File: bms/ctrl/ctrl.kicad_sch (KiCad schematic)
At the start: 72 parts

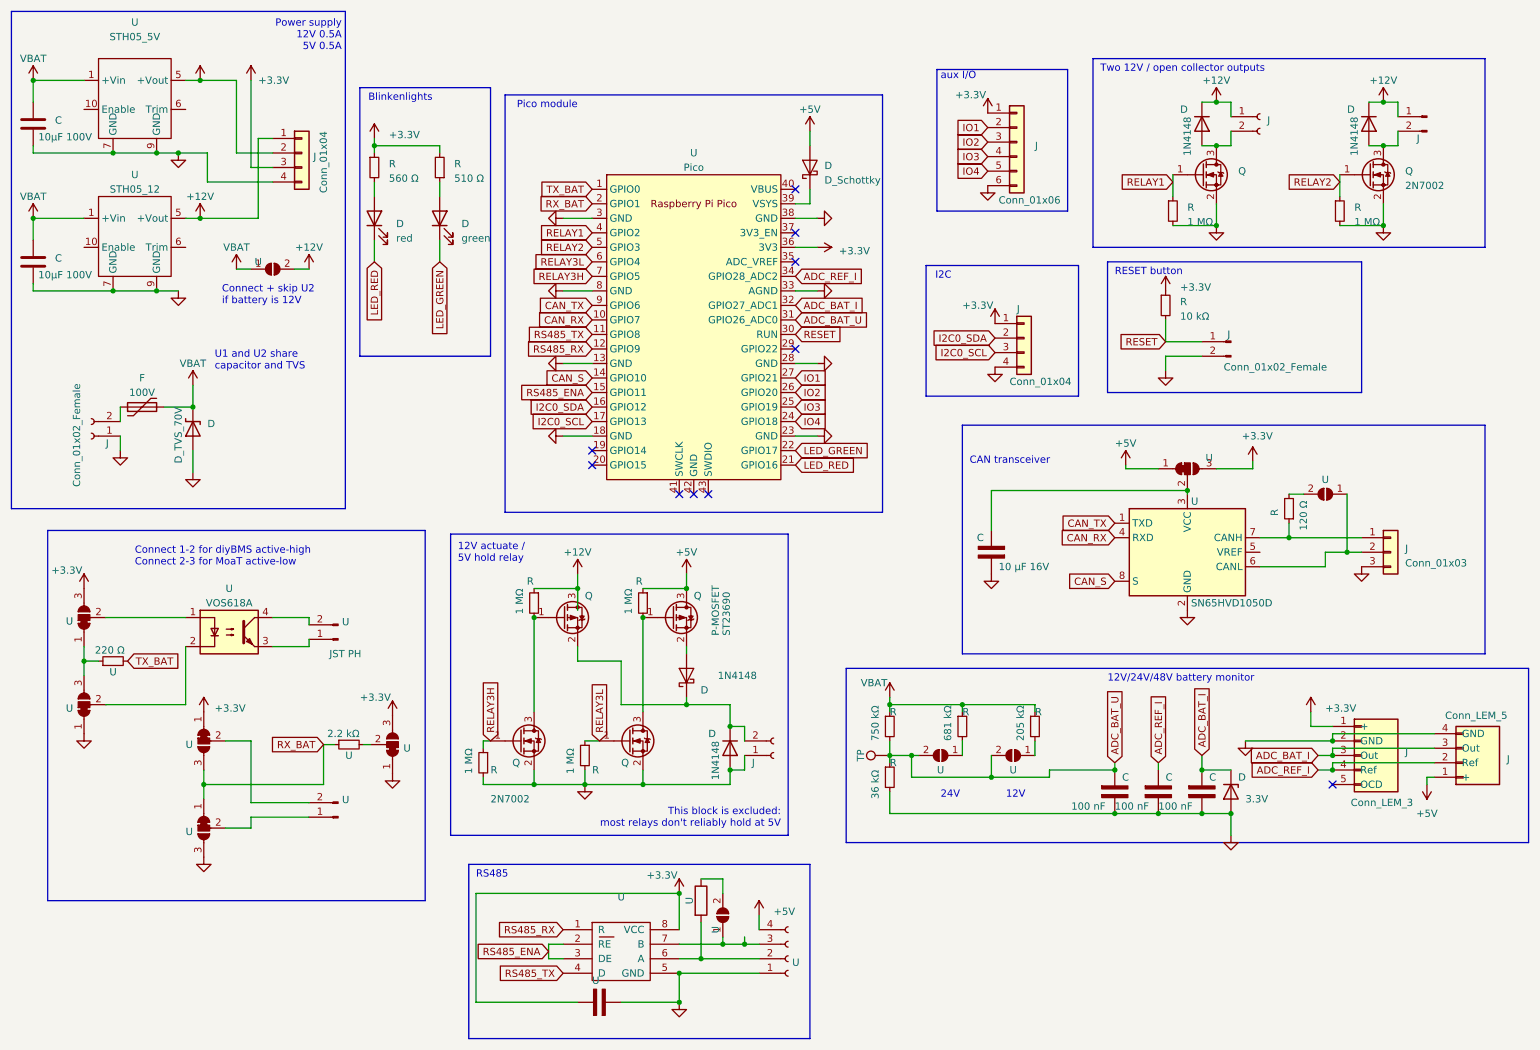
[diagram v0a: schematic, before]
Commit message: Old check-in: ctrl
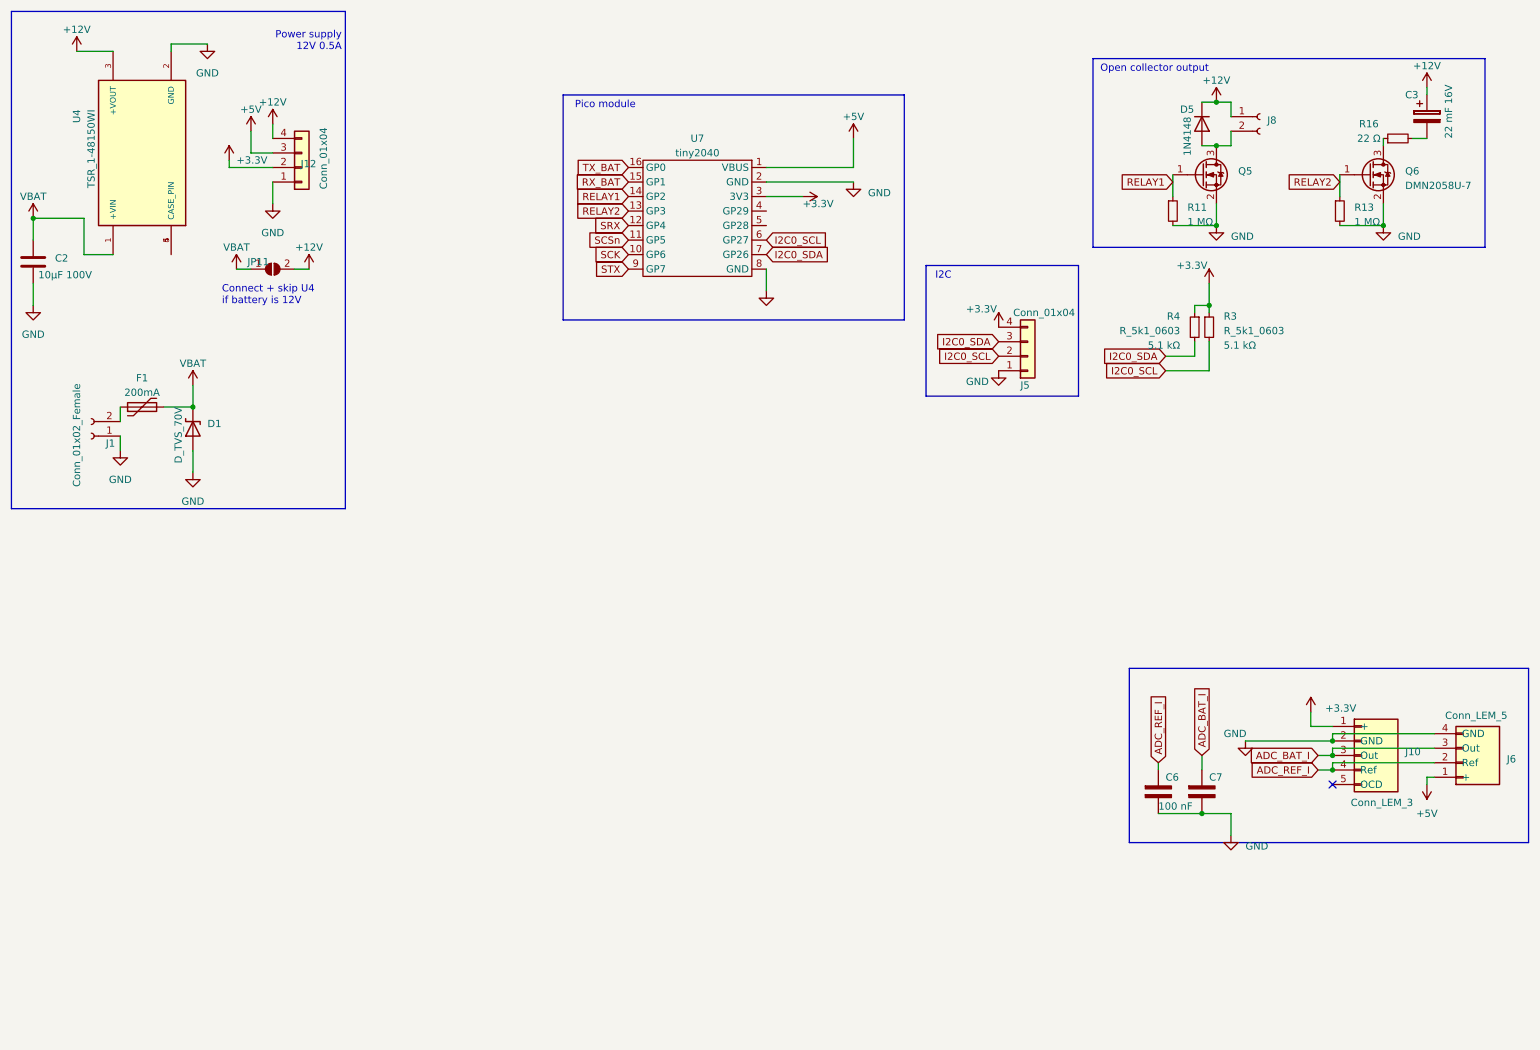
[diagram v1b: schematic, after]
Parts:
- removed C: CP_1µ_100V_0805, Resistor_SMD:R_0805_2012Metric, symbol localparts:CP_10µ_100V_1210
- removed C: CP_100n_50V_0603, Capacitor_SMD:C_0603_1608Metric, symbol localparts:CP_100n_50V_0603
- removed C: CP_10µ_16V_0603, Capacitor_SMD:C_0603_1608Metric, symbol localparts:CP_10µ_16V_0603
- removed D: LED_green, LED_SMD:LED_0805_2012Metric, symbol localparts:LED_green
- removed D: D_Zener_3V3, localstuff:SOD80, symbol localparts:D_Zener_3V3
- removed D: 1N4148, Diode_THT:D_DO-35_SOD27_P7.62mm_Horizontal, symbol localstuff:D_Schottky
- removed D (x2): 1N4148, Diode_THT:D_DO-35_SOD27_P7.62mm_Horizontal, symbol Diode:1N4148
- removed D: D_Schottky, symbol localstuff:D_Schottky
- removed D: LED_red, LED_SMD:LED_0805_2012Metric, symbol localparts:LED_red
- removed J: Conn_01x06, symbol Connector_Generic:Conn_01x06
- removed J: Conn_01x02_Female, symbol Connector:Conn_01x02_Female
- removed J (x2): Conn_01x02_Female, symbol Connector:Conn_01x02_Male
- removed J: Conn_01x03, symbol Connector_Generic:Conn_01x03
- removed Q (x2): ST23690, Package_DFN_QFN:AO_DFN-8-1EP_5.55x5.2mm_P1.27mm_EP4.12x4.6mm, symbol Transistor_FET:BSS83P
- removed Q (x2): 2N7002, Package_TO_SOT_SMD:SOT-23, symbol localparts:Q_NMOS_20V_4A_lowVth
- removed R: R_120_0603, Resistor_SMD:R_0603_1608Metric, symbol localparts:R_120_0603
- removed R: R_10k_0603, Resistor_SMD:R_0603_1608Metric, symbol localparts:R_10k_0603
- removed R: R_510_0603, Resistor_SMD:R_0603_1608Metric, symbol localparts:R_510_0603
- removed R (x4): R_1M_0603, Resistor_SMD:R_0603_1608Metric, symbol localparts:R_1M_0603
- removed R: R_36k_0603_1, Resistor_SMD:R_0603_1608Metric, symbol localparts:R_36k_0603_1
- removed R (x3): R_750k_0603, Resistor_SMD:R_0603_1608Metric, symbol localparts:R_750k_0603
- removed R: R_560_0603, Resistor_SMD:R_0603_1608Metric, symbol localparts:R_560_0603
- removed TP: TestPoint, symbol Connector:TestPoint
- removed U: SN65HVD1050D, Package_SO:SOIC-8_3.9x4.9mm_P1.27mm, symbol Interface_CAN_LIN:SN65HVD1050D
- removed U (x6): (no value), symbol Jumper:SolderJumper_3_Bridged12
- removed U (x4): (no value), symbol Jumper:SolderJumper_2_Open
- removed U: STH05_12, localstuff:STH05, symbol localstuff:STH05_12
- removed U: (no value), symbol ControllerCircuit:SN65HVD75DR
- removed U (x2): (no value), symbol Connector:Conn_01x02_Male
- removed U: (no value), symbol localparts:R_2k2_0603
- removed U: (no value), symbol Device:R
- removed U: (no value), symbol Connector:Conn_01x04_Female
- removed U: Pico, RPi_Pico:RPi_Pico_SMD_TH, symbol pico:Pico
- removed U: (no value), symbol localparts:R_220_0603
- removed U: (no value), symbol localparts:CP_100n_50V_0603
- removed U: VOS618A, Package_SO:SOP-4_4.4x2.6mm_P1.27mm, symbol localparts:VOS618A
- removed U: STH05_5V, localstuff:STH05, symbol localstuff:STH05_5V
- added C3: CP_22m_16V, Capacitor_THT:CP_Radial_D22.0mm_P10.00mm_SnapIn, symbol localparts:CP_22m_16V
- added R16: R_22_0603, Resistor_SMD:R_0603_1608Metric, symbol localparts:R_22_0603
- added R3, R4: R_5k1_0603, Resistor_SMD:R_0603_1608Metric, symbol localparts:R_5k1_0603
- added U4: TSR_1-48150WI, localstuff:TSR_1-48150WI, symbol localstuff:TSR_1-48150WI
- added U7: tiny2040, localstuff:tiny2040, symbol localstuff:tiny2040
- C2: renamed from C; footprint Resistor_SMD:R_0805_2012Metric -> Resistor_SMD:R_1210_3225Metric
- D5: renamed from D; footprint Diode_THT:D_DO-35_SOD27_P7.62mm_Horizontal -> Diode_SMD:D_SOD-123
- F1: renamed from F; value Polyfuse 100V -> Fuse; footprint Diode_SMD:D_SMA -> Fuse:Fuseholder_Cylinder-5x20mm_Stelvio-Kontek_PTF78_Horizontal_Open; Display 100V -> 200mA; Farnell 3945785 -> (none)
- J1, J8: renamed from J; footprint (none) -> localstuff:Conn_P5.0mm_2_Lumberg
- J12, J5: renamed from J; footprint (none) -> Connector_PinHeader_2.54mm:PinHeader_1x04_P2.54mm_Vertical
- JP11: renamed from U; value (none) -> Bat12V; footprint (none) -> Jumper:SolderJumper-2_P1.3mm_Open_RoundedPad1.0x1.5mm
- Q5, Q6: renamed from Q; value 2N7002 -> DMN2058U-7
- renumbered C to C6, C to C7, D to D1, J to J10, J to J6, R to R11, R to R13
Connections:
- net +12V: now also J12.4 (Pin_4), C3.1, U4.3 (+VOUT); no longer J12.1 (Pin_1)
- net +3V3: now also J12.2 (Pin_2), J5.4 (Pin_4), R3.1, R4.1, U7.3 (3V3); no longer J12.3 (Pin_3), J5.1 (Pin_1)
- net +5V: now also J12.3 (Pin_3), U7.1 (VBUS); no longer J12.2 (Pin_2)
- net GND: now also J12.1 (Pin_1), J5.1 (Pin_1), U4.2 (GND), U7.2 (GND), U7.8 (GND); no longer J12.4 (Pin_4), J5.4 (Pin_4)
- net I2C0_SCL: now also J5.2 (Pin_2), R3.2, U7.6 (GP27); no longer J5.3 (Pin_3)
- net I2C0_SDA: now also J5.3 (Pin_3), R4.2, U7.7 (GP26); no longer J5.2 (Pin_2)
- net RELAY1: now also U7.14 (GP2)
- net RELAY2: now also U7.13 (GP3)
- net RX_BAT: now also U7.15 (GP1)
- net TX_BAT: now also U7.16 (GP0)
- net VBAT: now also U4.1 (+VIN)
- net at Q6.3 (D): now also R16.1
- new net: U4.4 (CASE_PIN), U4.5 (CASE_PIN)
- new net: C3.2, R16.2
- new net SCK: U7.10 (GP6)
- new net SCSn: U7.11 (GP5)
- new net SRX: U7.12 (GP4)
- new net STX: U7.9 (GP7)
- no-connect marks 10 -> 1
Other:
- note added: "Connect + skip U4 if battery is 12V"
- note added: "Open collector output"
- note added: "Power supply 12V 0.5A"
- note removed: "12V"
- note removed: "12V actuate / 5V hold relay"
- note removed: "12V/24V/48V battery monitor"
- note removed: "24V"
- note removed: "Blinkenlights"
- note removed: "CAN transceiver"
- note removed: "Connect + skip U2 if battery is 12V"
- note removed: "Connect 1-2 for diyBMS active-high Connect 2-3 for MoaT active-low"
- note removed: "Power supply 12V 0.5A 5V 0.5A"
- note removed: "RESET button"
- note removed: "RS485"
- note removed: "This block is excluded: most relays don't reliably hold at 5V"
- note removed: "Two 12V / open collector outputs"
- note removed: "U1 and U2 share capacitor and TVS"
- note removed: "aux I/O"
- moved on the sheet: J5
